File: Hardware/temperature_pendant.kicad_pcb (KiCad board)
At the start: 2 copper layers, 38.1 x 25.4 mm, 5 parts, among them J1 CONN-6, SW1 SW-MOM, U1 BLINKM/MINM, U2 TMP3X

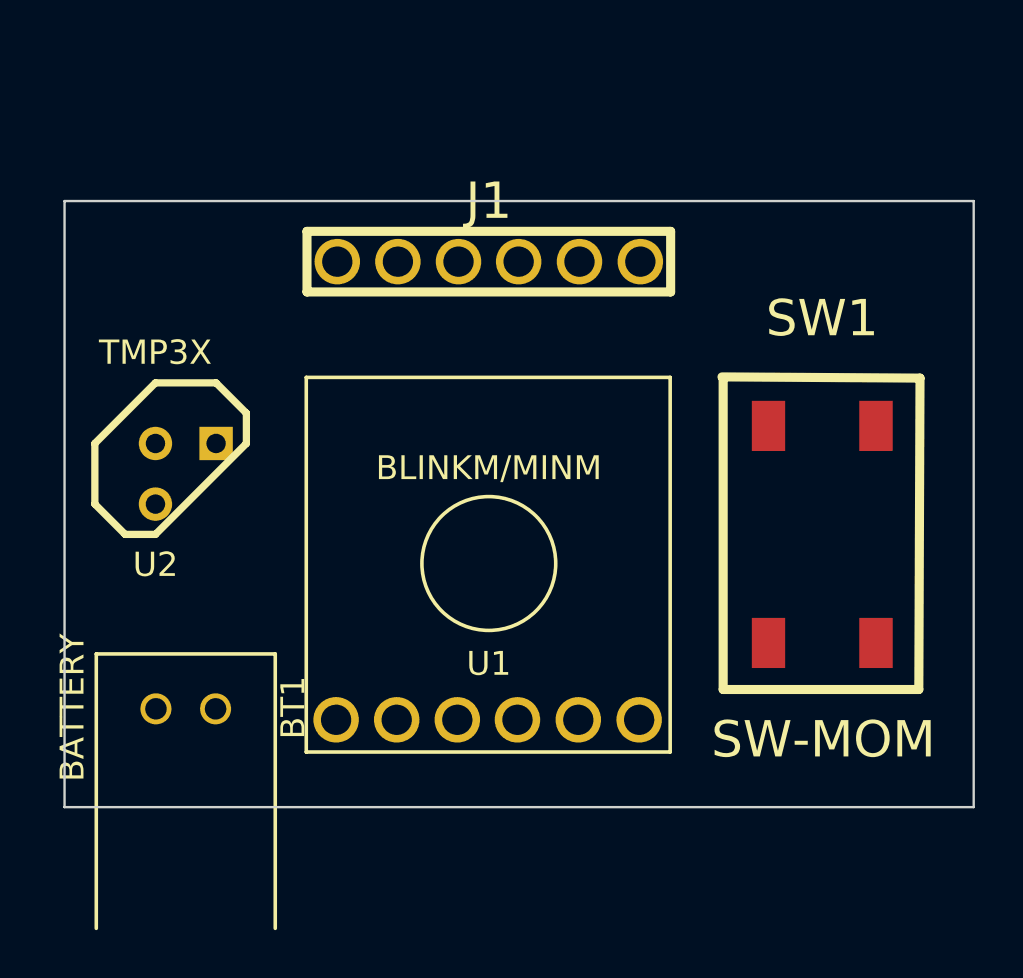
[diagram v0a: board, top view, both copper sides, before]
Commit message: Updated board
Updated board and first revision routing
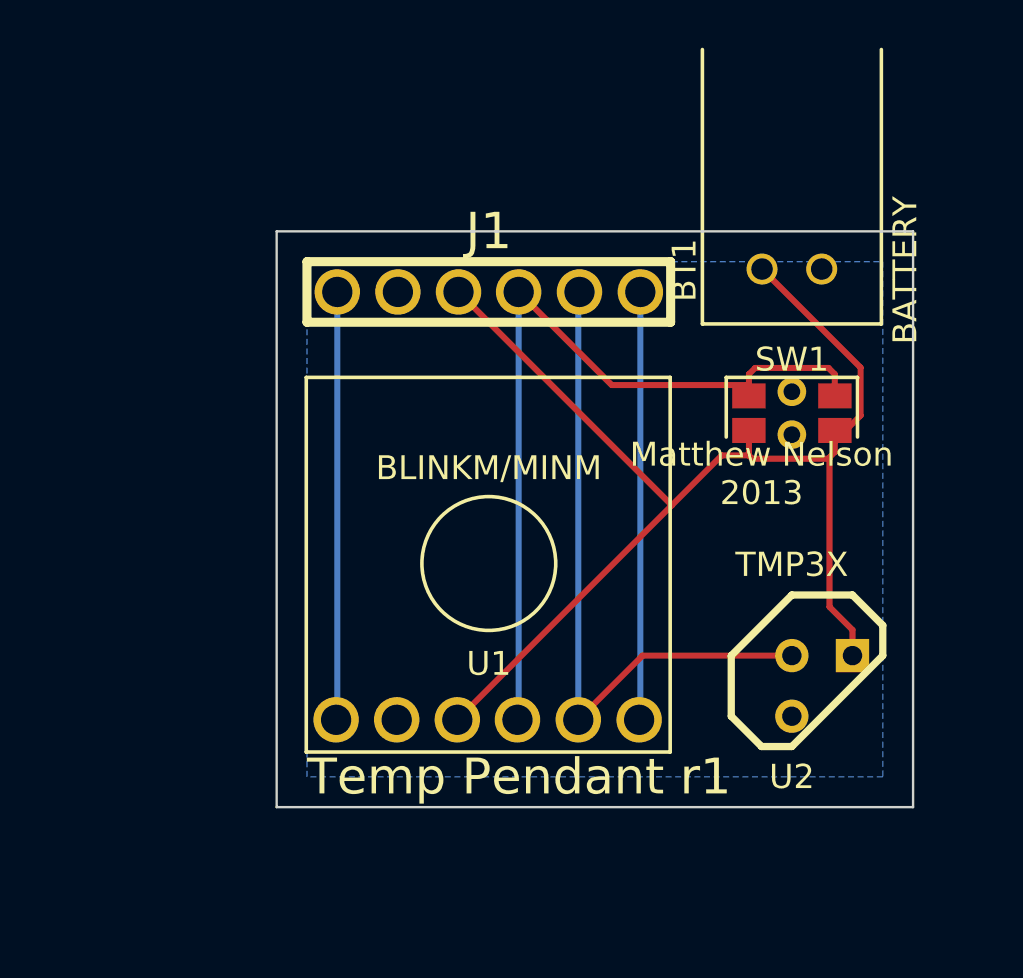
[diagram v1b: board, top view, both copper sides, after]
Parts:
- SW1: footprint SW_FSM4JSMATR -> SW-EVQP7
- moved BT1 44.7 mm to (221.0, 119.4), turned to 0 degrees
- moved U2 28.1 mm to (222.2, 146.1)
- moved SW1 5.24 mm to (221.0, 134.6)
- moved J1 1.27 mm to (208.3, 129.5)
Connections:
- J1 pad 1: (no net) -> RST
- J1 pad 2: (no net) -> GND
- J1 pad 3: (no net) -> +BATT
- J1 pad 4: (no net) -> SW
- J1 pad 5: (no net) -> TEMP
- J1 pad 6: (no net) -> MISO
- SW1 pad 1: (no net) -> SW
- SW1 pad 2: (no net) -> +BATT
- U1 pad 1: (no net) -> RST
- U1 pad 2: (no net) -> GND
- U1 pad 3: (no net) -> +BATT
- U1 pad 4: (no net) -> SW
- U1 pad 5: (no net) -> TEMP
- U1 pad 6: (no net) -> MISO
- U2 pad 1: (no net) -> +BATT
- U2 pad 2: (no net) -> TEMP
- U2 pad 3: (no net) -> GND
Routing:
- net +BATT: track 0.00 -> 53.2 mm
- net SW: track 0.00 -> 34.8 mm
- net TEMP: track 0.00 -> 28.0 mm
- net RST: track 0.00 -> 18.0 mm
- net MISO: track 0.00 -> 18.0 mm
- added copper zone on B.Cu, net GND
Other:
- board size 38.1 x 25.4 mm -> 26.7 x 24.1 mm
- board text added: "Matthew Nelson 2013"
- board text added: "Temp Pendant r1"
